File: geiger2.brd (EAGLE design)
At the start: 160 x 100 mm, 110 parts, among them Q1 IRF840, Q2 CSM-7X-DU, T1 BC847, T5 BC847, U1 STM32F042KXTX, U2 TPS562200DDCT, X1 22-23-2021, X2 22-23-2041, X3 22-23-2101, X4 22-23-2041

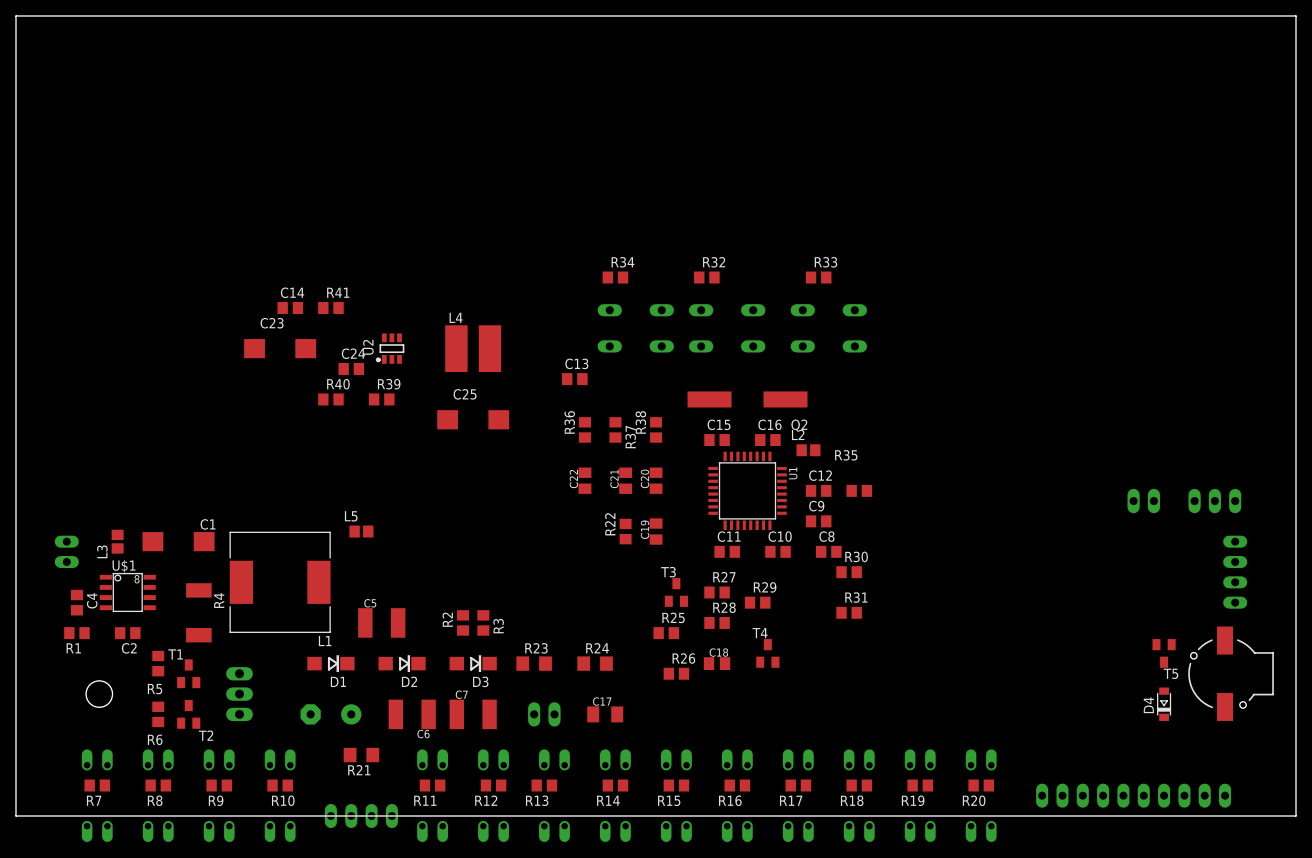
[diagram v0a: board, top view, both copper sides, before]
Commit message: Add routing
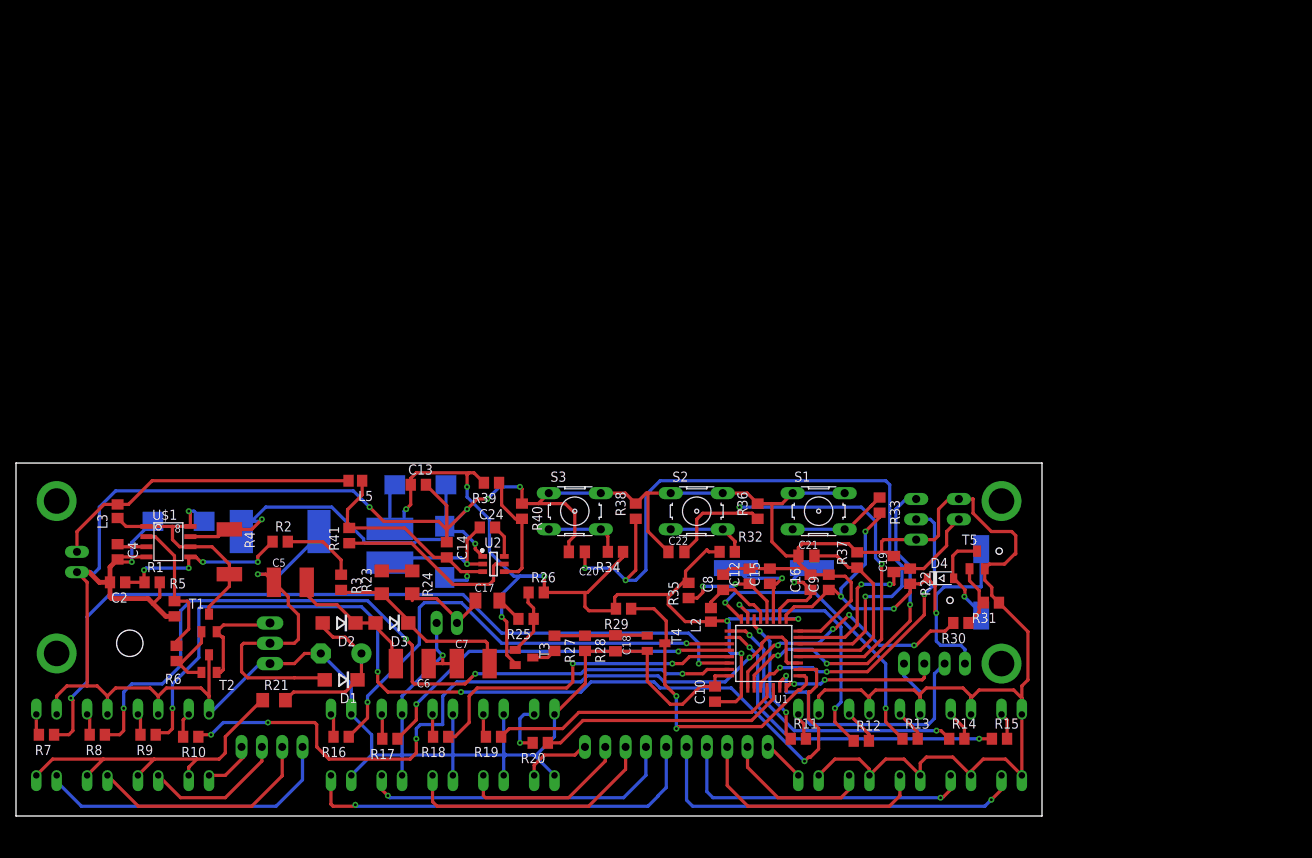
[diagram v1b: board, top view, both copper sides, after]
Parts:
- removed C11: (no value), rcl:C0805
- moved X3 57.5 mm to (82.5, 8.64), turned to 0 degrees
- moved R20 55.4 mm to (65.5, 9.14)
- moved OK14 55.0 mm to (66.0, 8.89)
- moved OK13 53.7 mm to (59.7, 8.89)
- moved R19 53.7 mm to (59.7, 9.91)
- moved R18 52.7 mm to (53.1, 9.91)
- moved OK12 52.5 mm to (53.3, 8.89)
- moved R17 51.4 mm to (46.7, 9.65)
- moved OK11 51.2 mm to (47.0, 8.89)
- moved OK10 49.9 mm to (40.6, 8.89)
- moved R16 49.9 mm to (40.6, 9.91)
- moved OK5 47.4 mm to (99.1, 8.89)
- moved R12 46.3 mm to (105.7, 9.40), turned to 0 degrees
- moved OK6 46.2 mm to (105.4, 8.89)
- moved R11 46.1 mm to (97.8, 9.65), turned to 0 degrees
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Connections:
- removed net N$38: OK5.3
- net +3V3: no longer C11.1
- net GND: now also OK5.3; no longer C11.2
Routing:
- net GND: track 0.00 -> 585.9 mm, vias 0 -> 7
- net +3V3: track 0.00 -> 194.6 mm, vias 0 -> 11
- net OK13: track 0.00 -> 123.7 mm, vias 0 -> 4
- net OK11: track 0.00 -> 104.3 mm, vias 0 -> 2
- net OK12: track 0.00 -> 100.0 mm, vias 0 -> 4
- net OK14: track 0.00 -> 93.2 mm, vias 0 -> 4
- net N$66: track 0.00 -> 91.7 mm, vias 0 -> 3
- net OK6: track 0.00 -> 61.0 mm, vias 0 -> 2
- net N$61: track 0.00 -> 57.9 mm, vias 0 -> 2
- net N$42: track 0.00 -> 51.9 mm, vias 0 -> 1
- net N$41: track 0.00 -> 49.0 mm, vias 0 -> 1
- net OK7: track 0.00 -> 47.2 mm, vias 0 -> 2
- net N$5: track 0.00 -> 43.9 mm, vias 0 -> 1
- net N$55: track 0.00 -> 43.1 mm, vias 0 -> 3
- net OK8: track 0.00 -> 42.6 mm, vias 0 -> 2
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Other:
- board size 160 x 100 mm -> 128.2 x 44.1 mm
